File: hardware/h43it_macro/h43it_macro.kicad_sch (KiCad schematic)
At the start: 25 parts, among them J1 Conn_01x04_Pin, SW1 SW_Push, SW2 SW_Push

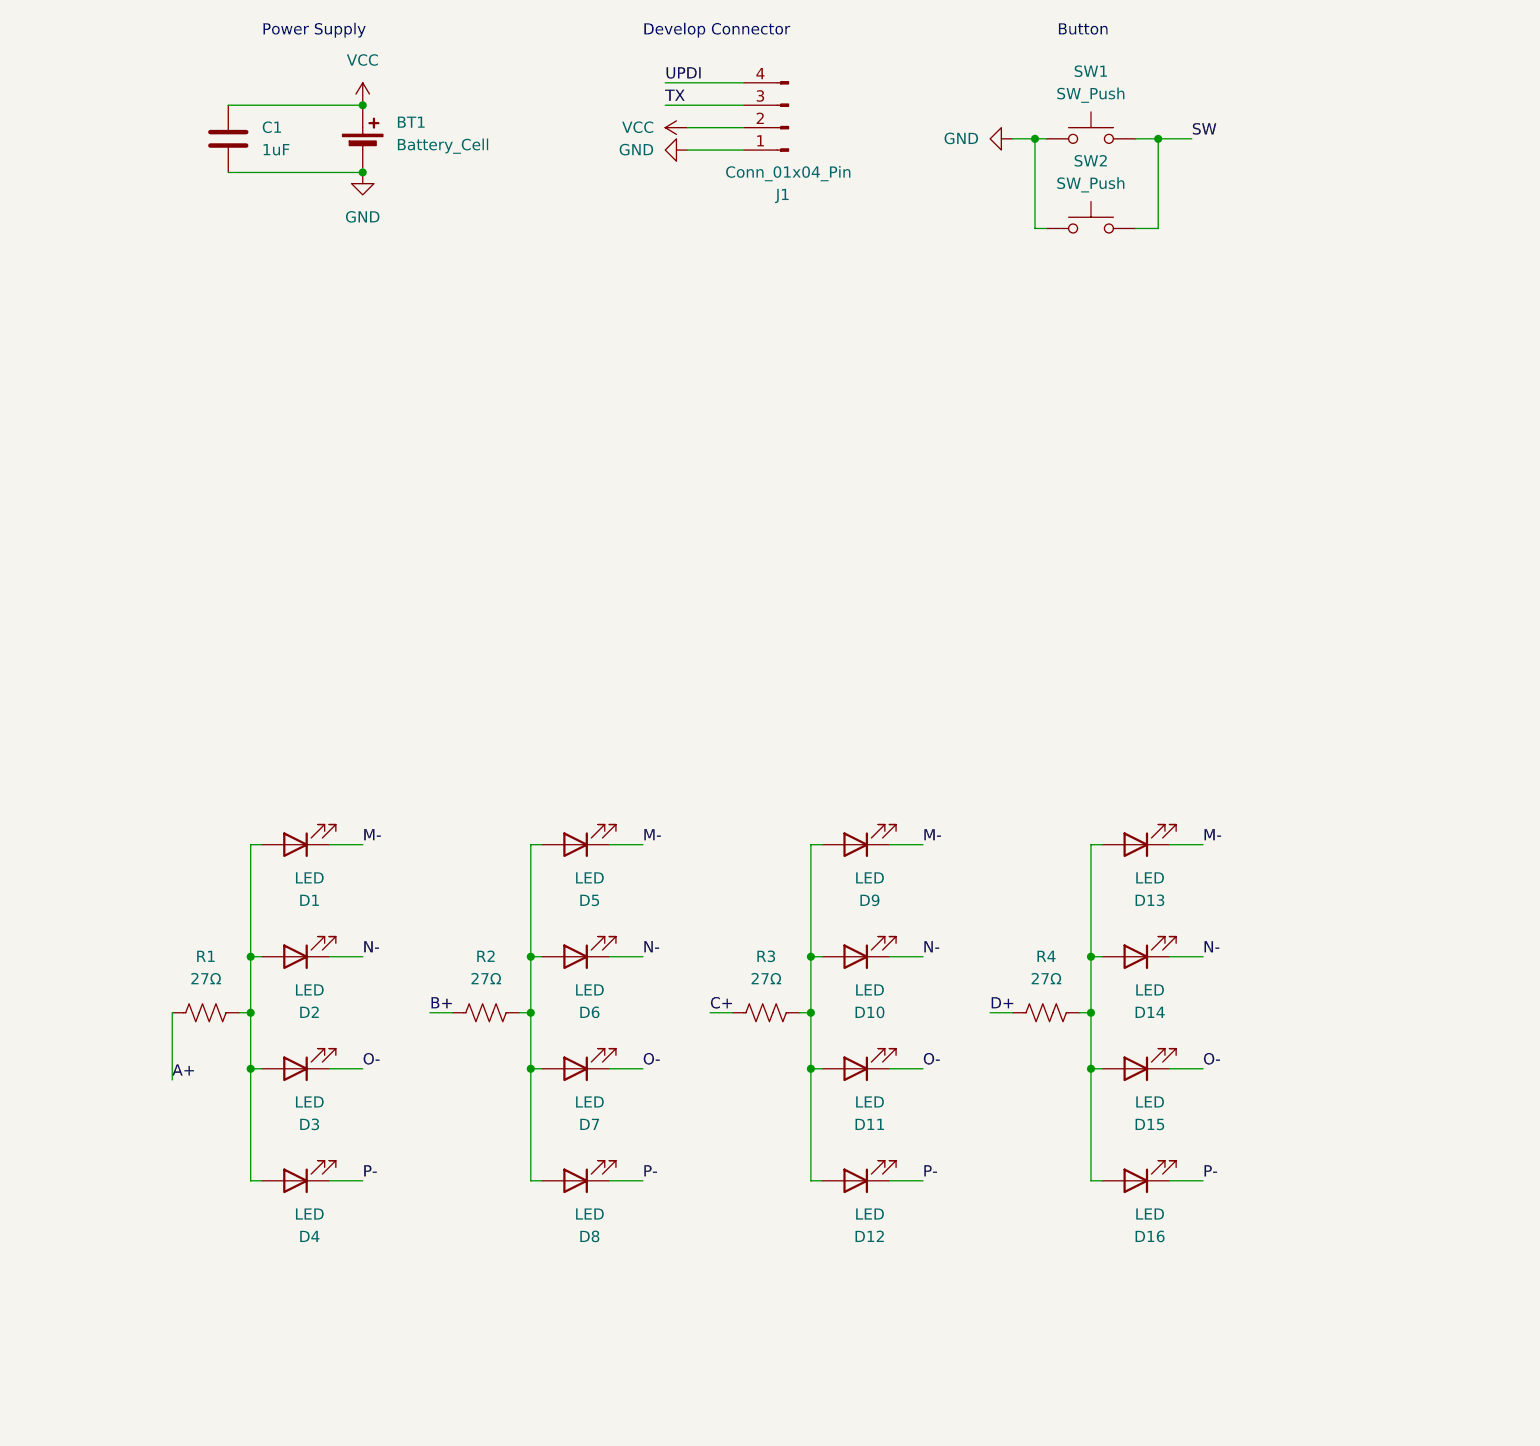
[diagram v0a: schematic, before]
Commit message: updates
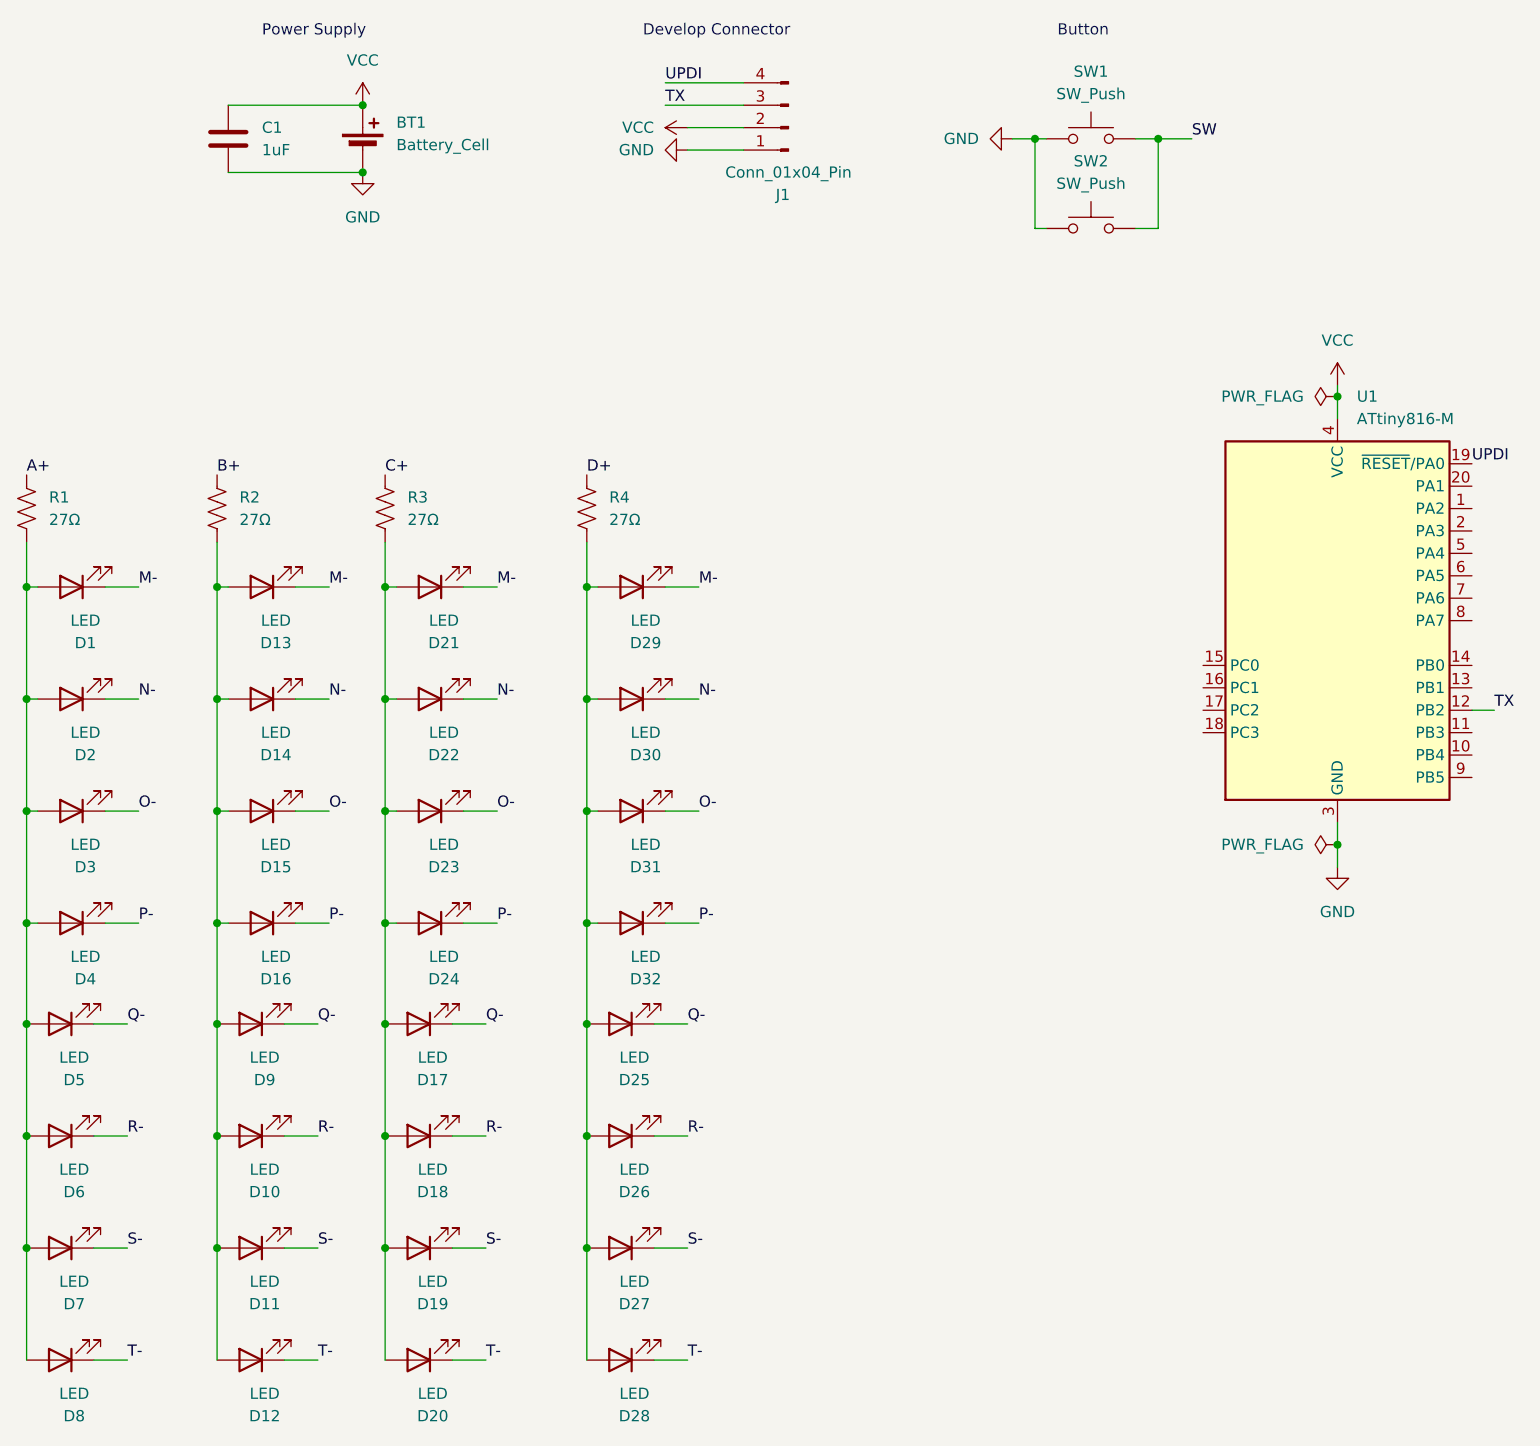
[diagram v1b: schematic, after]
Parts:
- added D17, D18, D19, D20, D21, D22, D23, D24, D25, D26, D27, D28, D29, D30, D31, D32: LED, LED_SMD:LED_0805_2012Metric, symbol Device:LED
- added U1: ATtiny816-M, Package_DFN_QFN:VQFN-20-1EP_3x3mm_P0.4mm_EP1.7x1.7mm, symbol MCU_Microchip_ATtiny:ATtiny816-M
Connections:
- net A+: now also R1.2; no longer R1.1
- net B+: now also R2.2; no longer R2.1
- net C+: now also R3.2; no longer R3.1
- net D+: now also R4.2; no longer R4.1
- net GND: now also U1.21 (GND), U1.3 (GND)
- net M-: now also D21.1 (K), D29.1 (K); no longer D5.1 (K), D9.1 (K)
- net N-: now also D22.1 (K), D30.1 (K); no longer D10.1 (K), D6.1 (K)
- net O-: now also D23.1 (K), D31.1 (K); no longer D11.1 (K), D7.1 (K)
- net P-: now also D24.1 (K), D32.1 (K); no longer D12.1 (K), D8.1 (K)
- net TX: now also U1.12 (PB2)
- net UPDI: now also U1.19 (~{RESET}/PA0)
- net VCC: now also U1.4 (VCC)
- net at D10.2 (A), D11.2 (A), D12.2 (A)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: now also D13.2 (A), D14.2 (A), D15.2 (A), D16.2 (A), R2.1; no longer R3.2
- net at D1.2 (A), D2.2 (A), D3.2 (A)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: now also D5.2 (A), D6.2 (A), D7.2 (A), D8.2 (A), R1.1; no longer R1.2
- new net: D17.2 (A), D18.2 (A), D19.2 (A), D20.2 (A), D21.2 (A), D22.2 (A), D23.2 (A), D24.2 (A), R3.1
- new net: D25.2 (A), D26.2 (A), D27.2 (A), D28.2 (A), D29.2 (A), D30.2 (A), D31.2 (A), D32.2 (A), R4.1
- new net Q-: D17.1 (K), D25.1 (K), D5.1 (K), D9.1 (K)
- new net R-: D10.1 (K), D18.1 (K), D26.1 (K), D6.1 (K)
- new net S-: D11.1 (K), D19.1 (K), D27.1 (K), D7.1 (K)
- new net T-: D12.1 (K), D20.1 (K), D28.1 (K), D8.1 (K)
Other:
- moved on the sheet: D1, D2, D3, D4, R1
